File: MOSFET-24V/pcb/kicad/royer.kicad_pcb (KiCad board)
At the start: 2 copper layers, 24 parts, among them J1 9-24V, J2 COIL, Q1 IRFB4410, Q2 IRFD110, Q3 IRFD110, Q4 IRFB4410

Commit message: net labels
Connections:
- net Net-(C1-Pad1) renamed /D1
- net Net-(C1-Pad2) renamed /C1
- net Net-(C3-Pad1) renamed /D2
- net Net-(C4-Pad2) renamed /C2
- net Net-(C5-Pad1) renamed /9V
- net Net-(D2-Pad1) renamed /X1
- net Net-(D3-Pad1) renamed /X2
- net Net-(J1-Pad2) renamed /24V
- net Net-(Q1-Pad1) renamed /G1
- net Net-(Q4-Pad1) renamed /G2

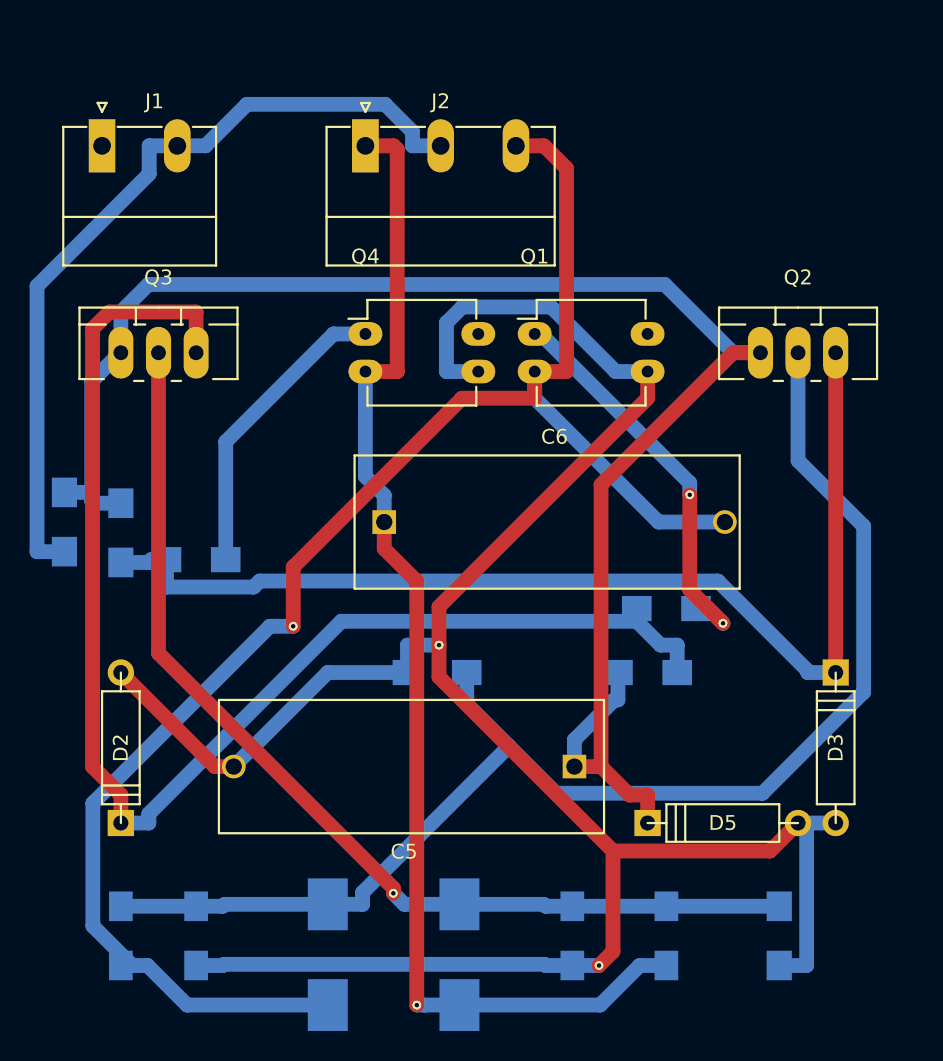
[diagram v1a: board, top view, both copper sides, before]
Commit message: rearranging SMD components
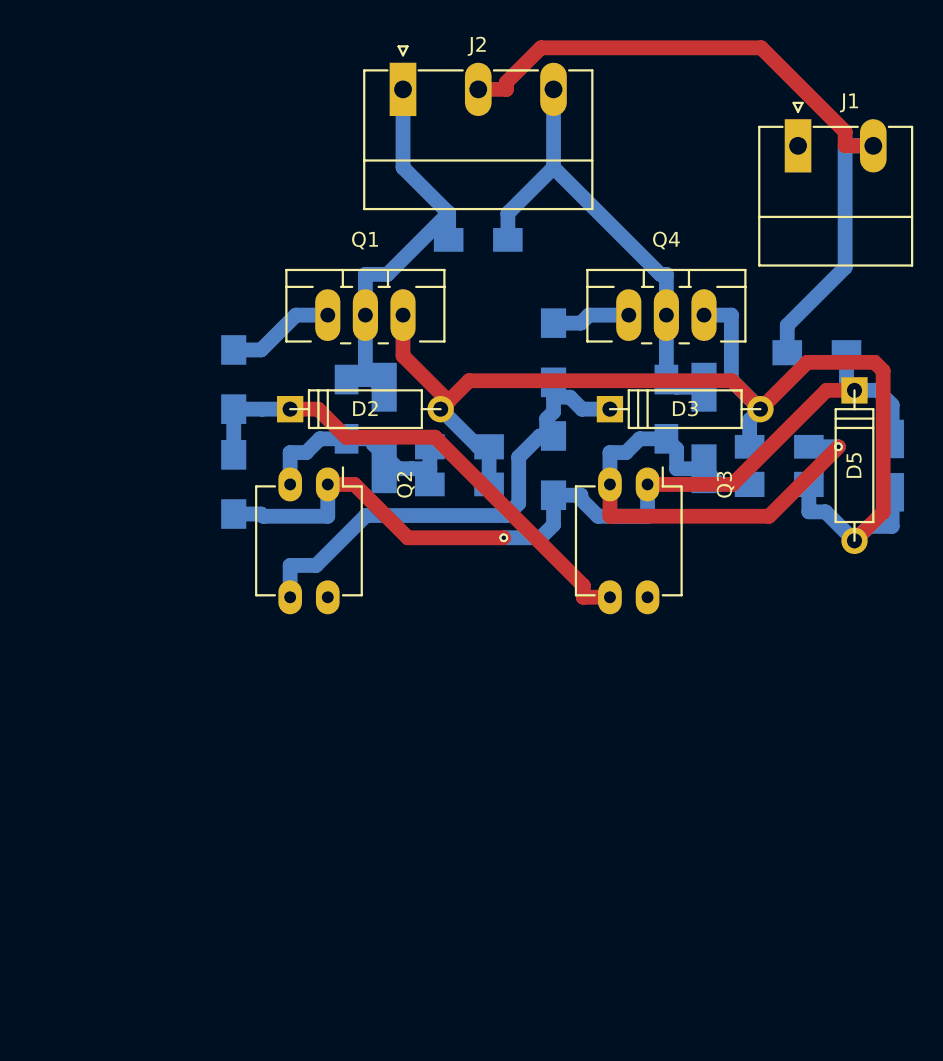
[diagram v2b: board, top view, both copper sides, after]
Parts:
- C5: footprint Capacitors_ThroughHole:C_Rect_L27_W9_H17_P23 -> Capacitors_SMD:c_elec_4x5.8; moved to B.Cu
- C6: footprint Capacitors_ThroughHole:C_Rect_L27_W9_H17_P23 -> Capacitors_SMD:C_1206_HandSoldering; moved to B.Cu
- D1, D4: footprint Diodes_SMD:MELF_Handsoldering -> Diodes_SMD:MiniMELF_Handsoldering
- Q1, Q4: footprint Housings_DIP:DIP-4_W7.62mm_LongPads -> TO_SOT_Packages_THT:TO-220_Neutral123_Vertical_LargePads
- Q2, Q3: footprint TO_SOT_Packages_THT:TO-220_Neutral123_Vertical_LargePads -> Housings_DIP:DIP-4_W7.62mm_LongPads
- moved R7 52.1 mm to (184.2, 57.1), turned to 0 degrees
- moved J1 47.0 mm to (182.9, 43.2)
- moved D4 39.2 mm to (176.5, 62.2), turned to 270 degrees
- moved C1 38.7 mm to (152.4, 61.0), turned to 90 degrees
- moved C3 35.9 mm to (181.6, 63.5), turned to 180 degrees
- moved D1 35.8 mm to (154.9, 62.2), turned to 270 degrees
- moved C4 35.6 mm to (174.0, 61.0), turned to 90 degrees
- moved C2 35.3 mm to (160.0, 66.0), turned to 0 degrees
- moved Q3 34.2 mm to (172.7, 66.0), turned to 270 degrees
- moved R2 33.0 mm to (144.8, 59.0), turned to 90 degrees
- moved Q2 33.0 mm to (151.1, 66.0), turned to 270 degrees
- moved R4 30.7 mm to (144.8, 66.0), turned to 90 degrees
- moved R5 30.5 mm to (181.6, 66.0), turned to 0 degrees
- moved R3 29.6 mm to (166.4, 64.8), turned to 90 degrees
- moved C5 29.5 mm to (189.2, 64.8), turned to 270 degrees
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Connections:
- J2 pad 1: /C2 -> /C1
- J2 pad 3: /C1 -> /C2
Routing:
- net /C1: track 110.6 -> 28.6 mm, vias 1 -> 0
- net /D1: track 90.1 -> 16.5 mm
- net GND: track 155.6 -> 82.1 mm, vias 2 -> 0
- net /X1: track 91.3 -> 34.2 mm
- net /9V: track 112.2 -> 61.7 mm, vias 0 -> 1
- net /C2: track 81.6 -> 31.9 mm, vias 1 -> 0
- net /X2: track 74.6 -> 33.3 mm
- net /D2: track 69.5 -> 35.5 mm
- net /G1: track 27.3 -> 7.32 mm, vias 2 -> 0
- net /G2: track 20.4 -> 5.30 mm
- net /24V: track 54.9 -> 48.9 mm
